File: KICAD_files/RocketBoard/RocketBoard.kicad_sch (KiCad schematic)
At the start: 24 parts, among them J1 GY-BME-280 Barometer, J5 PassiveBuzzer, K1 SRD-05VDC-SL-C, Q1 2N2222, SW1 RESET, SW2 ON/OFF, U1 RPI-Pico, U2 L7805, U3 ESP32-CAM

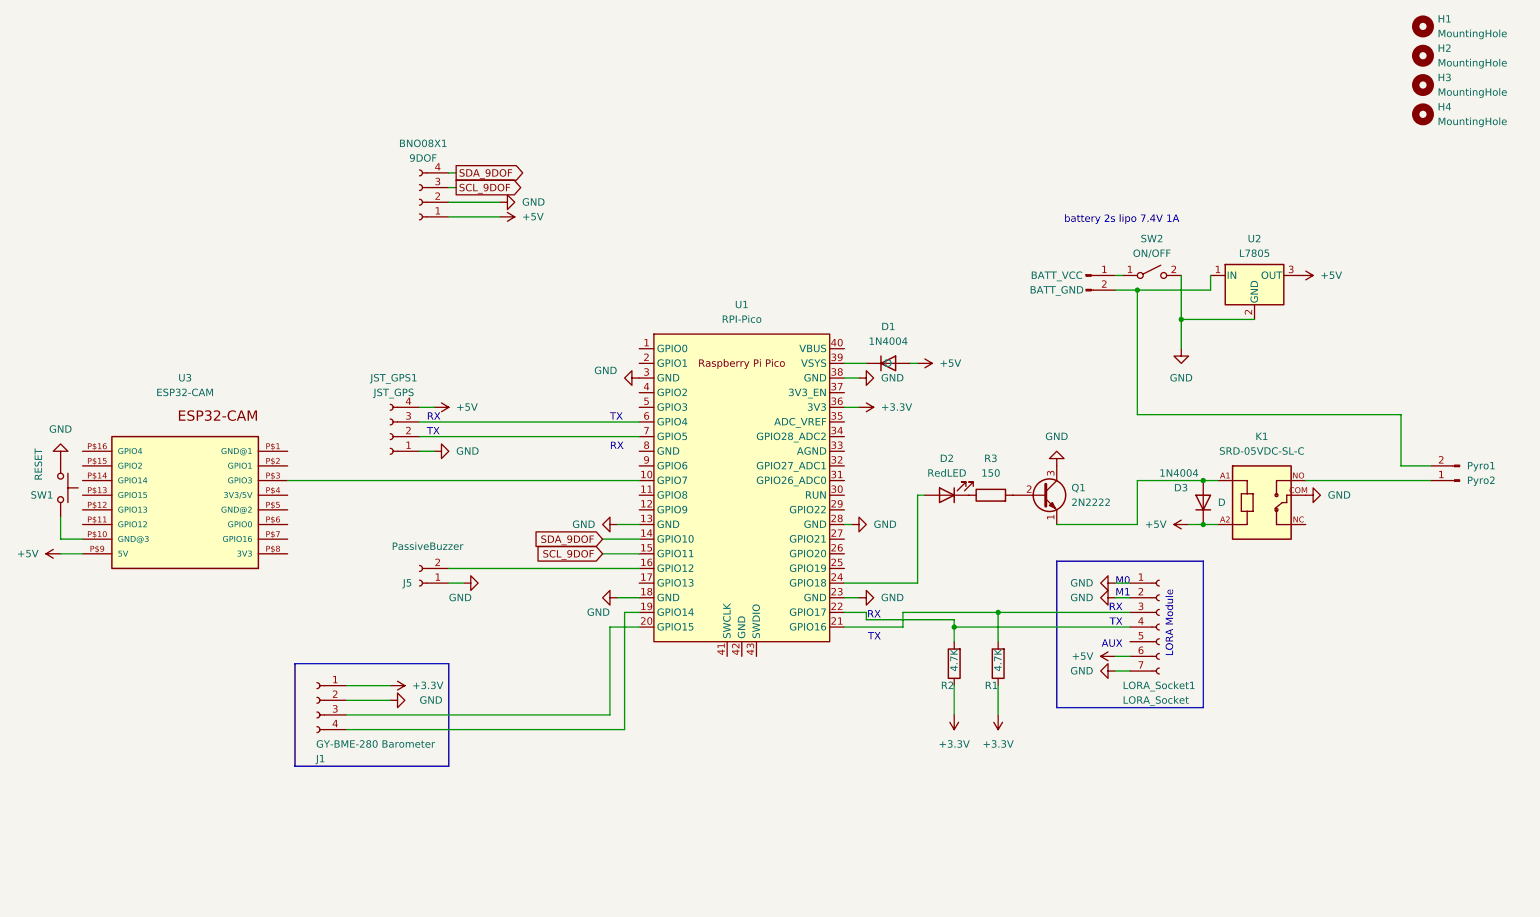
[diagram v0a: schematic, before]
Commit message: hhbh
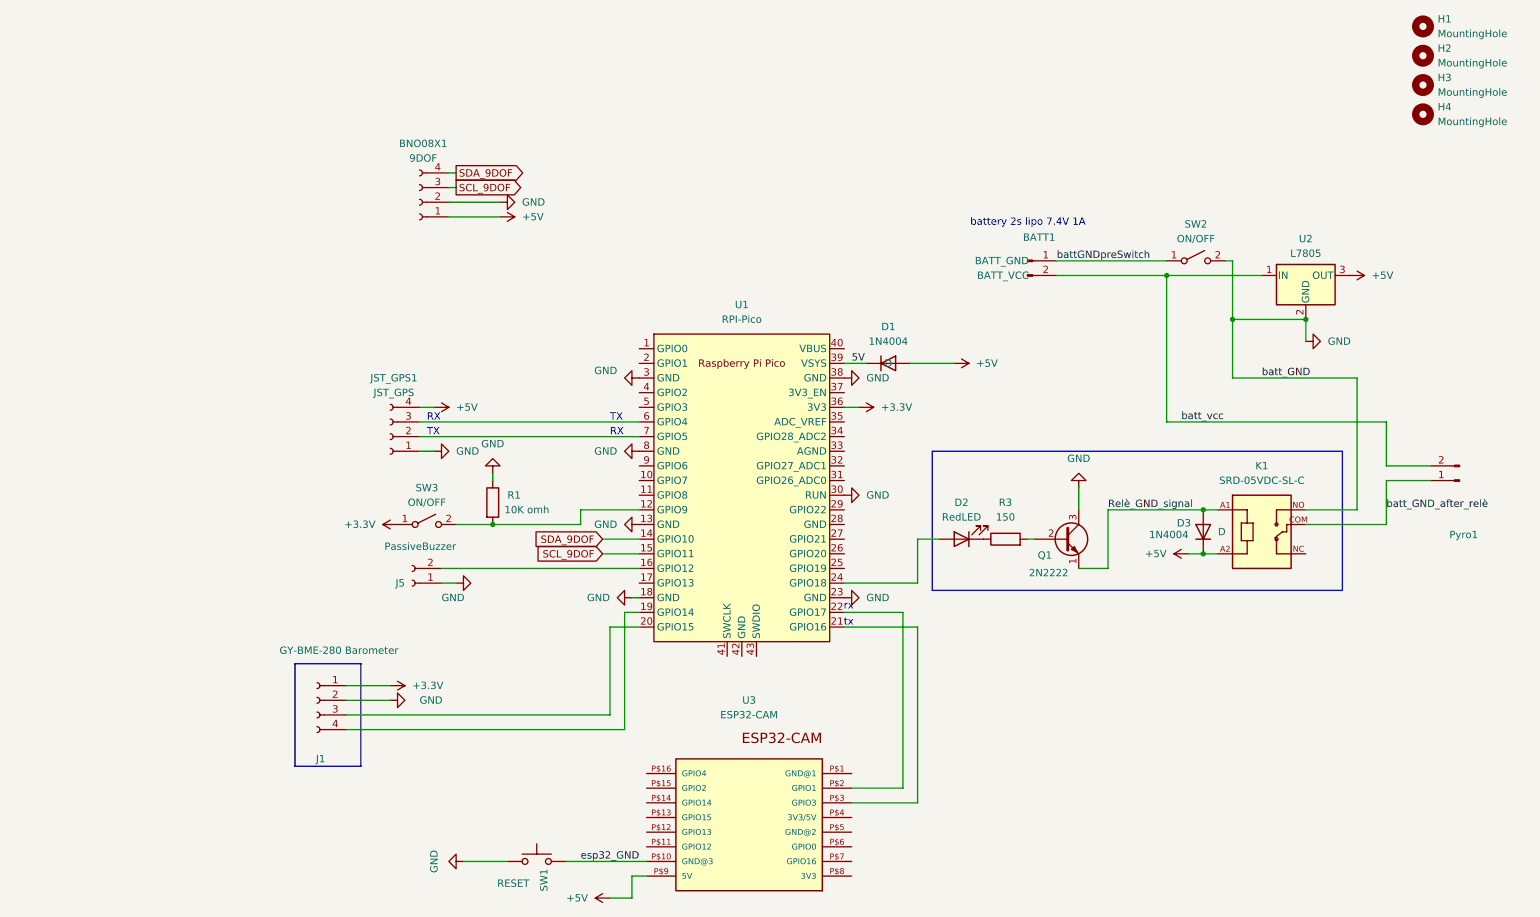
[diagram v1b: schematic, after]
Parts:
- removed LORA_Socket1: LORA_Socket, Connector_PinSocket_2.54mm:PinSocket_1x07_P2.54mm_Vertical, symbol Connector:Conn_01x07_Socket
- removed R2: 4.7K, Resistor_THT:R_Axial_DIN0207_L6.3mm_D2.5mm_P10.16mm_Horizontal, symbol Device:R
- added SW3: ON/OFF, roba_mia:Schiebeschalter SS-12D00, symbol Switch:SW_SPST
- BATT1: renamed from BATT_VCC; value BATT_GND -> ~
- H1, H2, H3, H4: footprint (none) -> MountingHole:MountingHole_2.1mm
- J5: footprint Buzzer_Beeper:Buzzer_TDK_PS1240P02BT_D12.2mm_H6.5mm -> roba_mia:myBuzzer
- K1: footprint Relay5V:RELAY_SRD-05VDC-SL-C -> roba_mia:ssr-41FDA
- Pyro1: value Pyro2 -> ~
- R1: value 4.7K -> 10K omh; footprint Resistor_THT:R_Axial_DIN0207_L6.3mm_D2.5mm_P10.16mm_Horizontal -> Resistor_THT:R_Axial_DIN0204_L3.6mm_D1.6mm_P5.08mm_Horizontal
- U1: footprint MCU_RaspberryPi_and_Boards:RPi_Pico_SMD_TH_2 -> raspberry pi pico:RPi_Pico_SMD_TH
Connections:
- net +3.3V: now also SW3.1 (A); no longer R1.1
- net GND: now also K1.NO, R1.1, U1.30 (RUN), U1.8 (GND); no longer K1.COM, U1.28 (GND)
- net batt_vcc: now reaches BATT1.2 (BATT_VCC), Pyro1.2 (Pin_2), U2.1 (IN)
- net battGNDpreSwitch: now reaches BATT1.1 (BATT_GND), SW2.1 (A)
- net at R1.2: now also U1.12 (GPIO9), SW3.2 (B); no longer U1.21 (GPIO16)
- net batt_GND_after_relè: now reaches Pyro1.1 (Pin_1)
- net batt_GND_after_relè: now also K1.COM; no longer K1.NO
- net at U1.10 (GPIO7): no longer U3.P$3 (GPIO3)
- net at U1.22 (GPIO17): now also U3.P$2 (GPIO1)
- net 5V : now reaches D1.1 (K), U1.39 (VSYS)
- net esp32_GND: now reaches SW1.2, U3.P$10 (GND@3)
- net Relè_GND_signal: now reaches D3.2 (A), K1.A1, Q1.1 (E)
- new net: U1.21 (GPIO16), U3.P$3 (GPIO3)
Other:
- note added: "rx"
- note added: "tx"
- note removed: "AUX"
- note removed: "LORA Module"
- note removed: "M0 M1"
- moved on the sheet: D2, D3, J5, K1, Q1, R3, SW1, SW2, U2, U3
